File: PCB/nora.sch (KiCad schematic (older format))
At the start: 218 parts, among them J1 USB_C_Receptacle_USB2.0, J2 Conn_01x04, J3 Conn_01x02, J5 Conn_02x03_Odd_Even, U1 ATmega32U4-MU, U2 24LC64, U4 Pico, Y1 16MHz

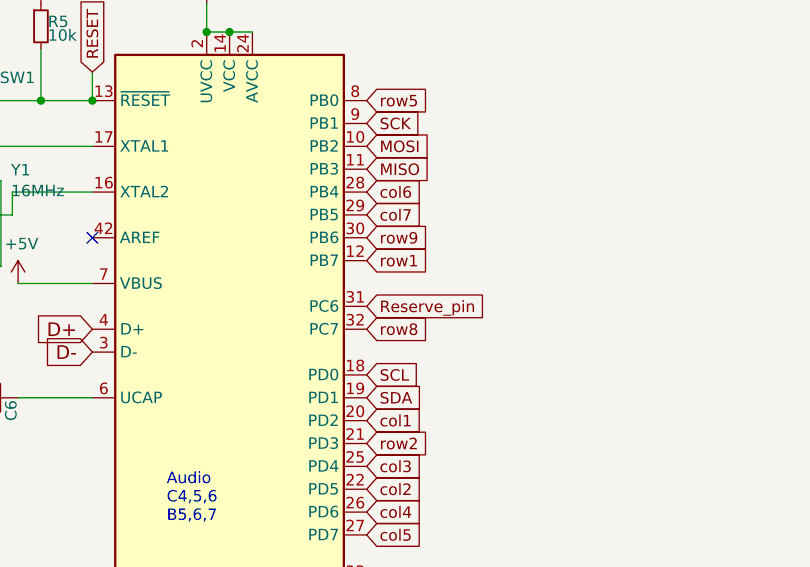
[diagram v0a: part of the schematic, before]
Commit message: WIP 怪しそうなところを配線中
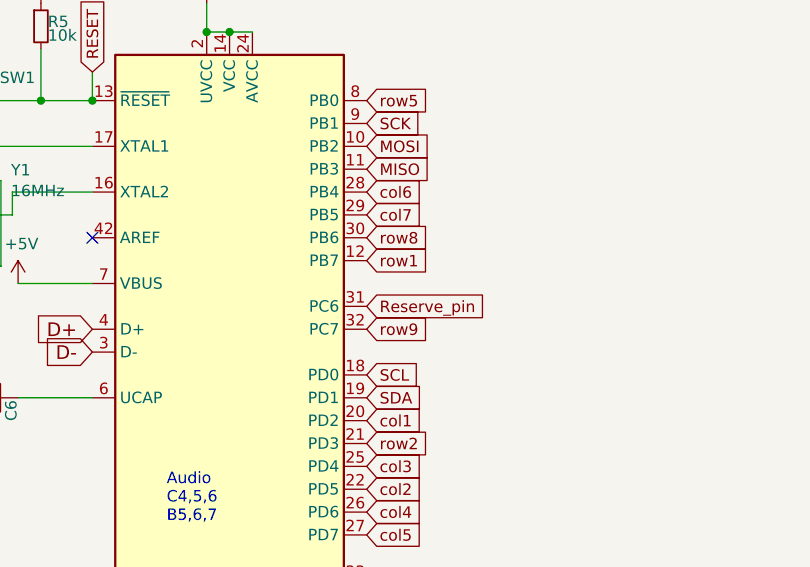
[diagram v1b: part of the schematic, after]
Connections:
- net row8: now also U1.30 (PB6); no longer U1.32 (PC7)
- net row9: now also U1.32 (PC7); no longer U1.30 (PB6)
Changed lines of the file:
@@
 Text GLabel 15325 2575 2    50   Input ~ 0
 row1
-Text GLabel 15325 2875 2    50   Input ~ 0
+Text GLabel 15325 2475 2    50   Input ~ 0
 row8
 Text GLabel 15325 1875 2    50   Input ~ 0
 row5
-Text GLabel 15325 2475 2    50   Input ~ 0
+Text GLabel 15325 2875 2    50   Input ~ 0
 row9
 Text GLabel 15325 2275 2    50   Input ~ 0
